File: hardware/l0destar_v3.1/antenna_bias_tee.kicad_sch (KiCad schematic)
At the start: 12 parts

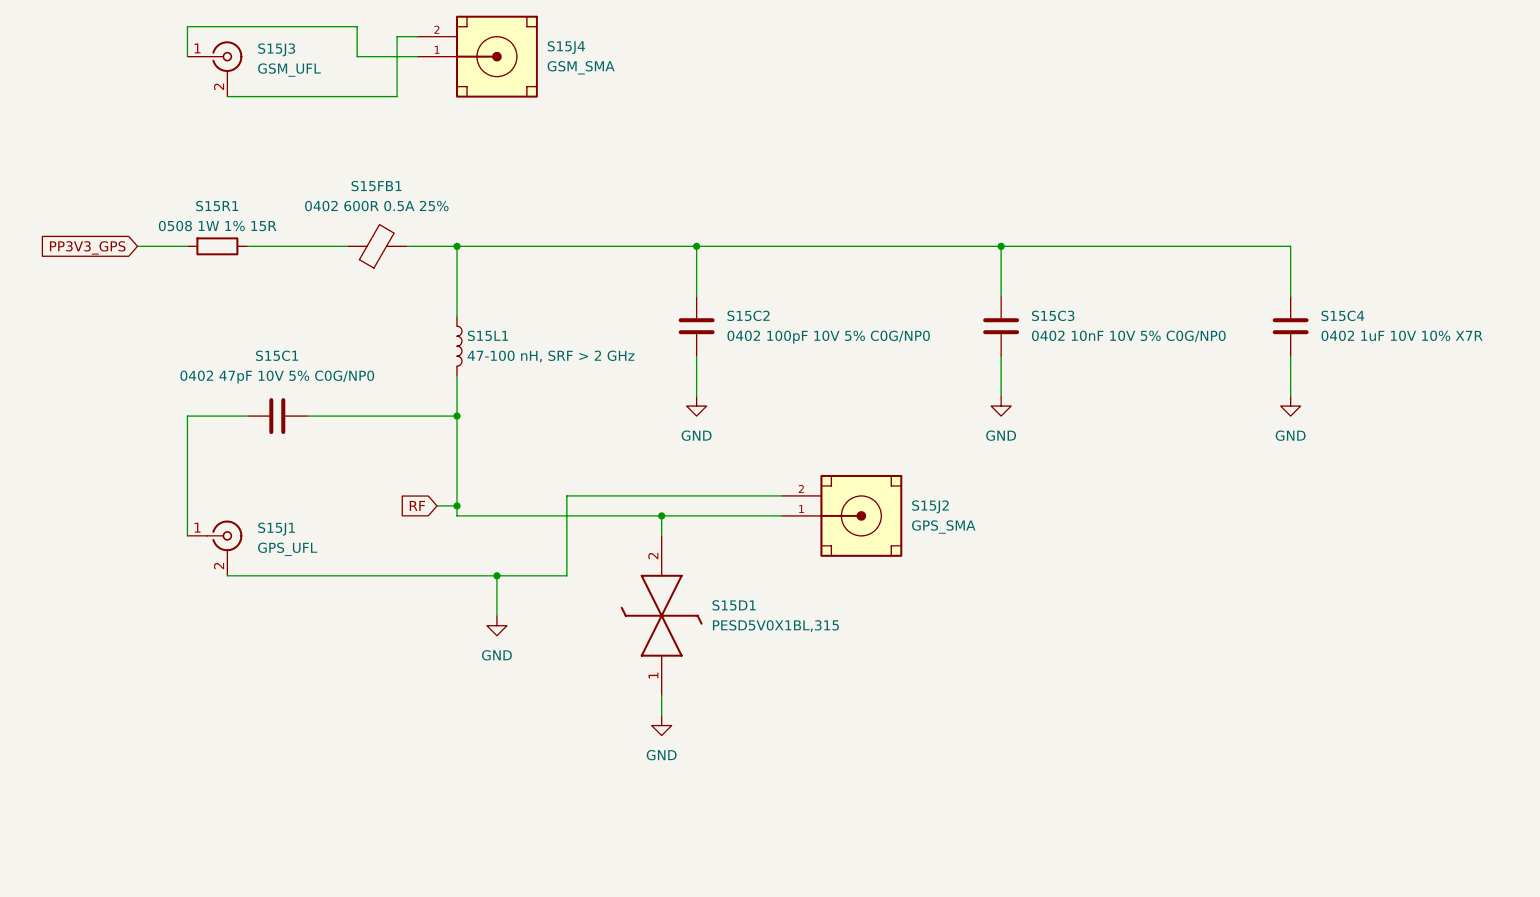
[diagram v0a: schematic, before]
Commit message: update v3.1
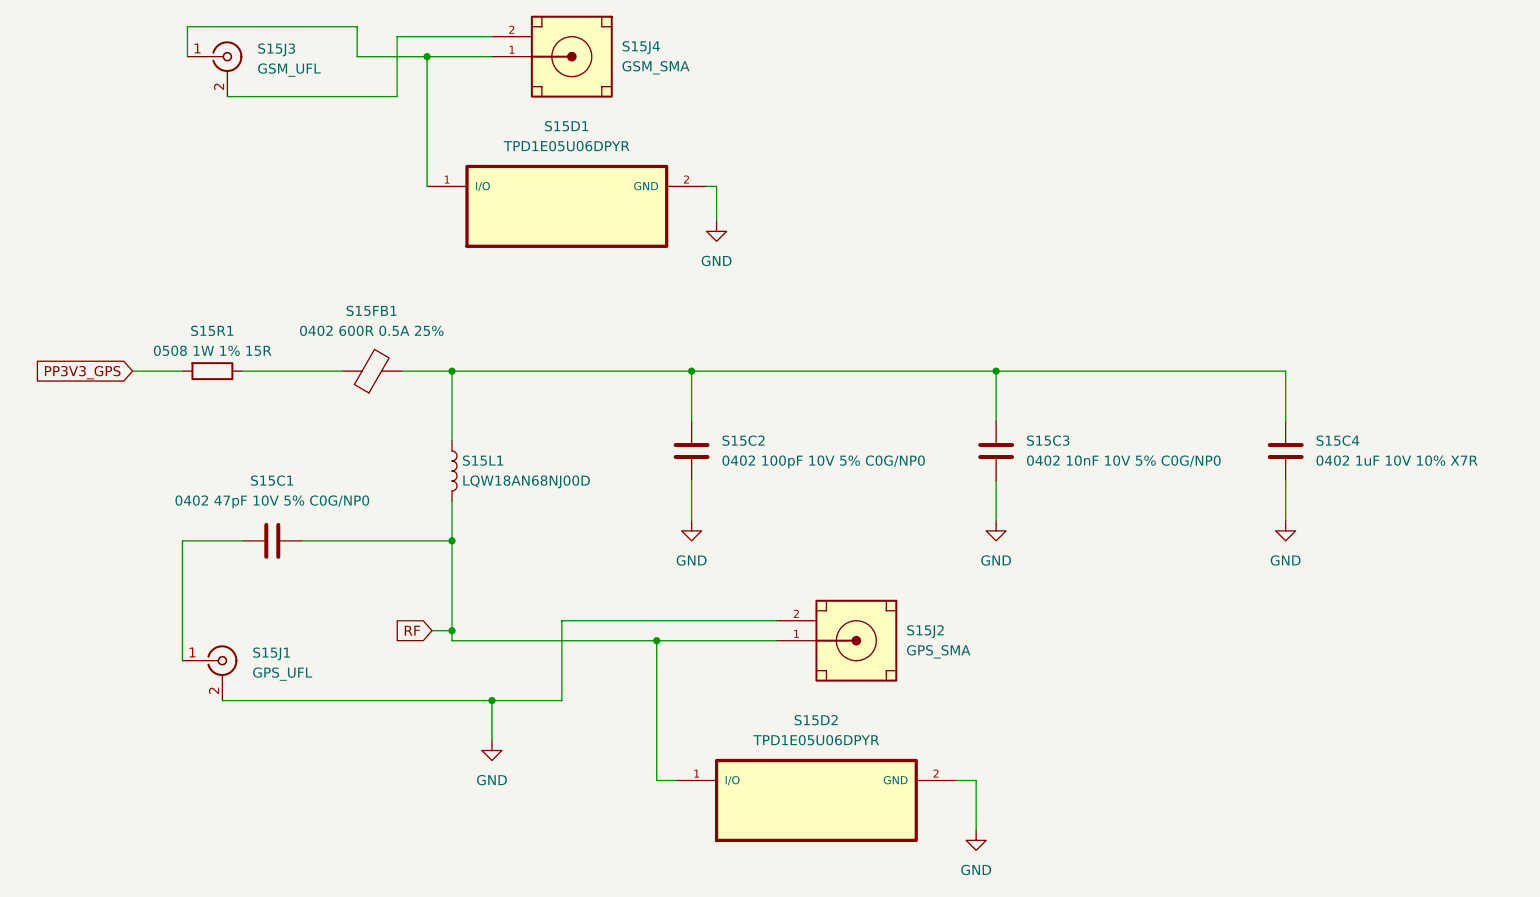
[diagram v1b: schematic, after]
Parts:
- removed S15D1: PESD5V0X1BL,315, libs:PESD5V0S1BL315, symbol PESD5V0X1BL_315:PESD5V0X1BL,315
- added S15D1, S15D2: TPD1E05U06DPYR, libs:DIO_TPD1E05U06DPYR, symbol TPD1E05U06DPYR:TPD1E05U06DPYR
- S15L1: value 47-100 nH, SRF > 2 GHz -> LQW18AN68NJ00D
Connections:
- net GND: now also S15D1.2 (GND), S15D2.2 (GND)
- net RF: now also S15D2.1 (I/O)
- net at S15J3.1 (In), S15J4.1: now also S15D1.1 (I/O)
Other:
- moved on the sheet: S15C1, S15C2, S15C3, S15C4, S15FB1, S15J1, S15J2, S15J4, S15L1, S15R1

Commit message: update v3.1
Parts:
- S15C1: Manufacturer_Name (none) -> Multicomp Pro; Manufacturer_Part_Number (none) -> 0402N470F500CT
- S15C2: Manufacturer_Name (none) -> Yageo; Manufacturer_Part_Number (none) -> AC0402FRNPO9BN101
- S15C3: Manufacturer_Name (none) -> Murata; Manufacturer_Part_Number (none) -> GRM1555CYA103JE01D
- S15C4: Manufacturer_Name (none) -> Kyocera AVX; Manufacturer_Part_Number (none) -> KAM05CR71A105KH
- S15D1, S15D2: Availability In Stock -> (none); Check_prices https://www.snapeda.com/parts/TPD1E05U06DPYR/Texas+Instrume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 -> (none); MF Texas Instruments -> (none); MP TPD1E05U06DPYR -> (none); Manufacturer_Name (none) -> Texas Instruments; Manufacturer_Part_Number (none) -> TPD1E05U06DPYR; Package X1SON-2 Texas Instruments -> (none); Price None -> (none); SnapEDA_Link https://www.snapeda.com/parts/TPD1E05U06DPYR/Texas+Instrume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 -> (none)
- S15FB1: Manufacturer_Name (none) -> Murata; Manufacturer_Part_Number (none) -> BLM15PX601SZ1D
- S15J1, S15J3: Manufacturer_Name (none) -> Hirose; Manufacturer_Part_Number (none) -> U.FL-R-SMT(01)
- S15J2, S15J4: Availability In Stock -> (none); Check_prices https://www.snapeda.com/parts/SMA-J-P-H-RA-TH1/Samtec+Inc./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 -> (none); MF Samtec -> (none); MP SMA-J-P-H-RA-TH1 -> (none); Manufacturer_Name (none) -> Samtec; Manufacturer_Part_Number (none) -> SMA-J-P-H-RA-TH1; Package None -> (none); Price None -> (none); Purchase-URL https://www.snapeda.com/api/url_track_click_mouser/?unipart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 -> (none); SnapEDA_Link https://www.snapeda.com/parts/SMA-J-P-H-RA-TH1/Samtec+Inc./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 -> (none)
- S15L1: Manufacturer_Name (none) -> Murata; Manufacturer_Part_Number (none) -> LQW18AN68NJ00D
- S15R1: Manufacturer_Name (none) -> CGS / TE Connectivity; Manufacturer_Part_Number (none) -> 3430A2F15RTDF
